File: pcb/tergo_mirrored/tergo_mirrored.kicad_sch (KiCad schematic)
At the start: 111 parts, among them J1 MJ-4PP-9, Q1 2N7002, SW1 SW_RESET, SW10 SW_PUSH, SW11 SW_PUSH, SW12 SW_PUSH, SW13 SW_PUSH, SW14 SW_PUSH, SW15 SW_PUSH, SW16 SW_PUSH, SW17 SW_PUSH, SW18 SW_PUSH, SW19 SW_PUSH, SW2 SW_PUSH, SW20 SW_PUSH, SW21 SW_PUSH, SW22 SW_PUSH, SW23 SW_PUSH, SW24 SW_PUSH, SW25 SW_PUSH, SW26 SW_PUSH, SW27 SW_PUSH, SW28 SW_PUSH, SW29 SW_PUSH, SW3 SW_PUSH, SW4 SW_PUSH, SW5 SW_PUSH, SW6 SW_PUSH, SW7 SW_PUSH, SW8 SW_PUSH, SW9 SW_PUSH, U1 Raspberry_Pi_Pico

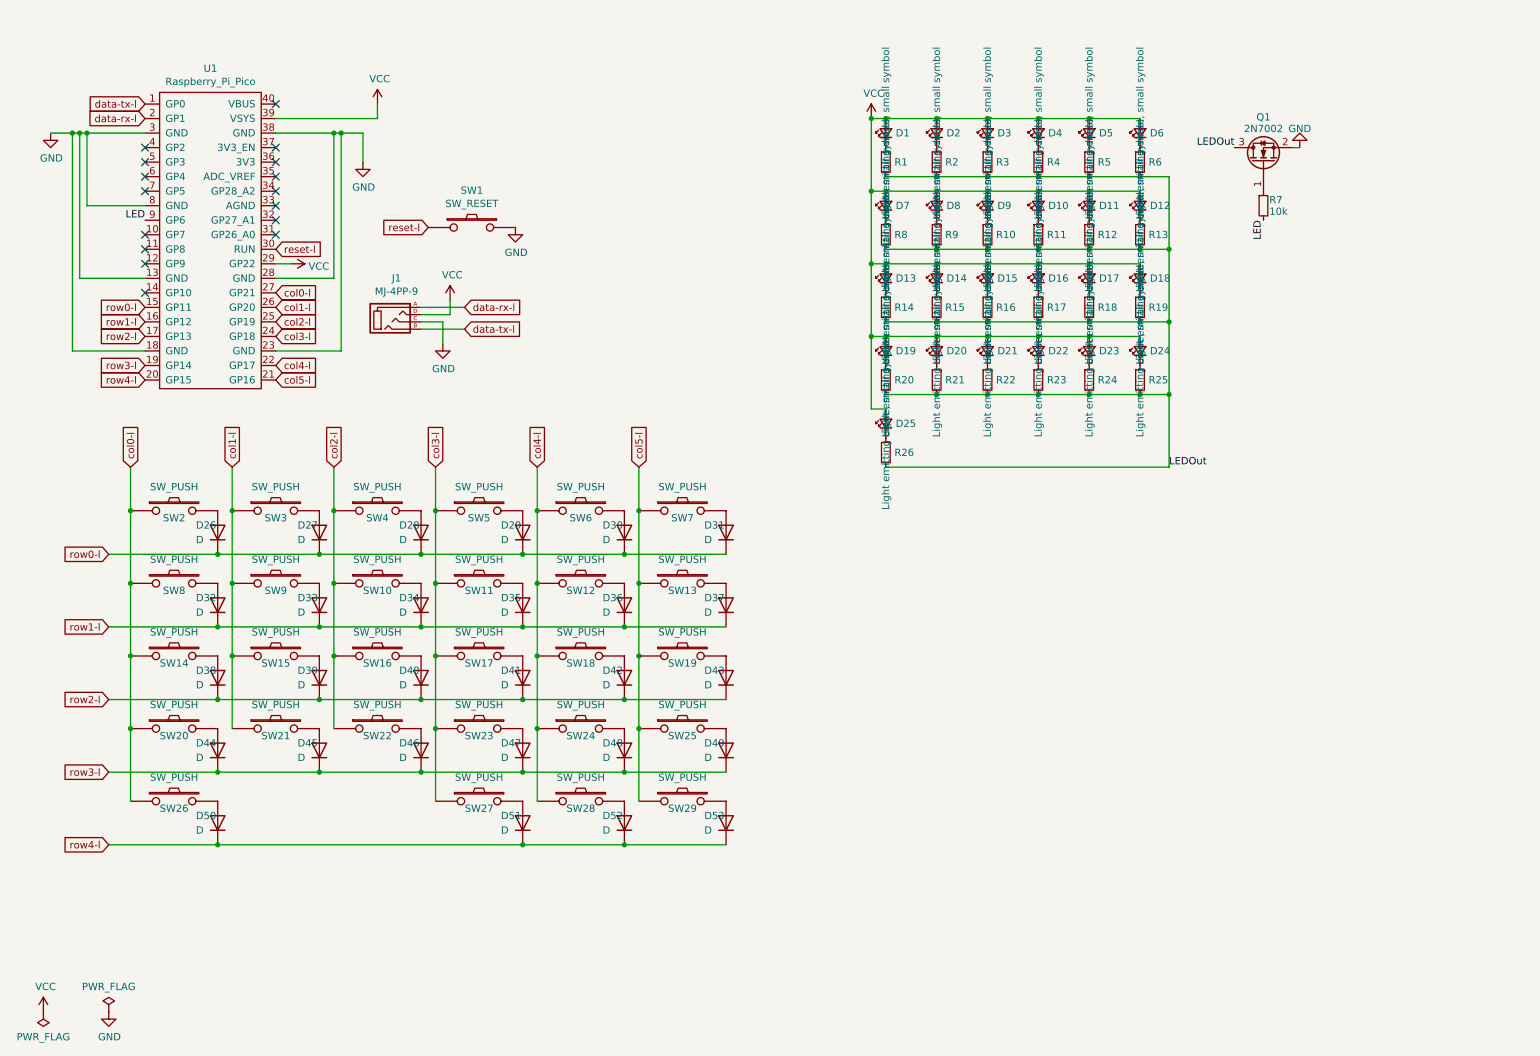
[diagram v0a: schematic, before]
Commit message: wip
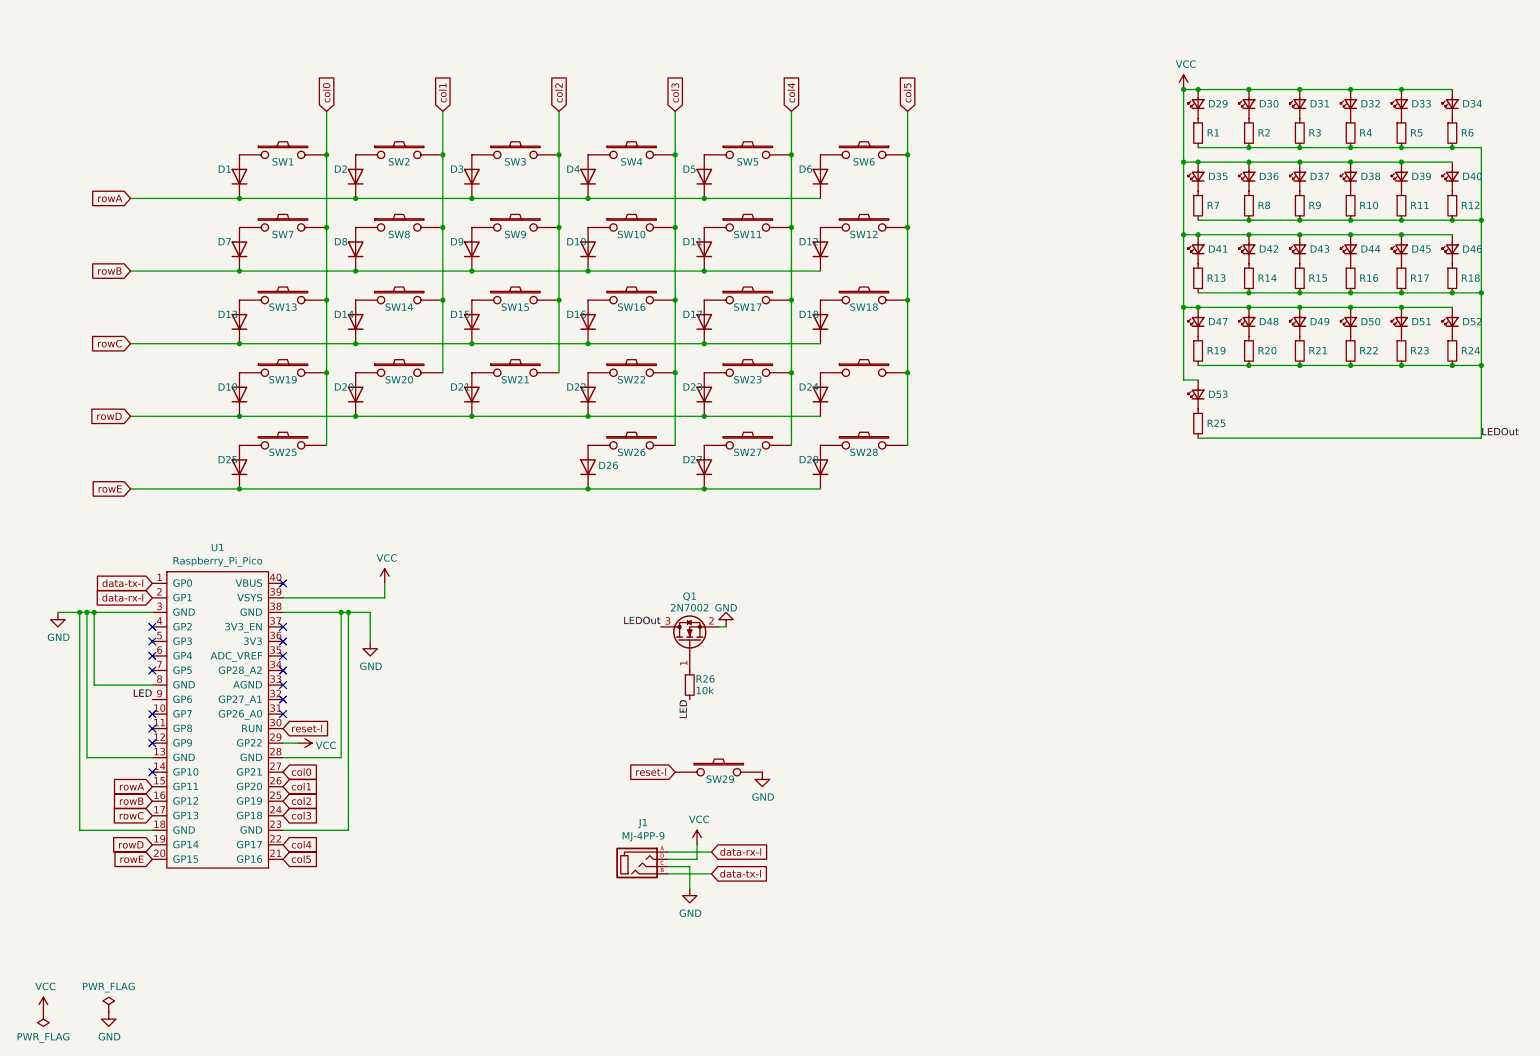
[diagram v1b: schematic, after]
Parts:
- D1: renamed from D26; value D -> 1n4148
- D10: renamed from D35; value D -> 1n4148
- D11: renamed from D36; value D -> 1n4148
- D12: renamed from D37; value D -> 1n4148
- D13: renamed from D38; value D -> 1n4148
- D14: renamed from D39; value D -> 1n4148
- D15: renamed from D40; value D -> 1n4148
- D16: renamed from D41; value D -> 1n4148
- D17: renamed from D42; value D -> 1n4148
- D18: renamed from D43; value D -> 1n4148
- D19: renamed from D44; value D -> 1n4148
- D2: renamed from D27; value D -> 1n4148
- D20: renamed from D45; value D -> 1n4148
- D21: renamed from D46; value D -> 1n4148
- D22: renamed from D47; value D -> 1n4148
- D23: renamed from D48; value D -> 1n4148
- D24: renamed from D49; value D -> 1n4148
- D25: renamed from D50; value D -> 1n4148
- D26: renamed from D51; value D -> 1n4148
- D27: renamed from D52; value D -> 1n4148
- D28: renamed from D53; value D -> 1n4148
- D3: renamed from D28; value D -> 1n4148
- D4: renamed from D29; value D -> 1n4148
- D5: renamed from D30; value D -> 1n4148
- D6: renamed from D31; value D -> 1n4148
- D7: renamed from D32; value D -> 1n4148
- D8: renamed from D33; value D -> 1n4148
- D9: renamed from D34; value D -> 1n4148
- SW1: renamed from SW2; footprint _tergo_lib:CherryMX_Choco_Hotswap -> _tergo_lib:SW_Hotswap_Kailh_MX_Plated_mirrored2_1.00u
- SW10: renamed from SW11; footprint _tergo_lib:CherryMX_Choco_Hotswap -> _tergo_lib:SW_Hotswap_Kailh_MX_Plated_mirrored2_1.00u
- SW11: renamed from SW12; footprint _tergo_lib:CherryMX_Choco_Hotswap -> _tergo_lib:SW_Hotswap_Kailh_MX_Plated_mirrored2_1.00u
- SW12: renamed from SW13; footprint _tergo_lib:CherryMX_Choco_Hotswap -> _tergo_lib:SW_Hotswap_Kailh_MX_Plated_mirrored2_1.00u
- SW13: renamed from SW14; footprint _tergo_lib:CherryMX_Choco_Hotswap -> _tergo_lib:SW_Hotswap_Kailh_MX_Plated_mirrored2_1.00u
- SW14: renamed from SW15; footprint _tergo_lib:CherryMX_Choco_Hotswap -> _tergo_lib:SW_Hotswap_Kailh_MX_Plated_mirrored2_1.00u
- SW15: renamed from SW16; footprint _tergo_lib:CherryMX_Choco_Hotswap -> _tergo_lib:SW_Hotswap_Kailh_MX_Plated_mirrored2_1.00u
- SW16: renamed from SW17; footprint _tergo_lib:CherryMX_Choco_Hotswap -> _tergo_lib:SW_Hotswap_Kailh_MX_Plated_mirrored2_1.00u
- SW17: renamed from SW18; footprint _tergo_lib:CherryMX_Choco_Hotswap -> _tergo_lib:SW_Hotswap_Kailh_MX_Plated_mirrored2_1.00u
- SW18: renamed from SW19; footprint _tergo_lib:CherryMX_Choco_Hotswap -> _tergo_lib:SW_Hotswap_Kailh_MX_Plated_mirrored2_1.00u
- SW19: renamed from SW20; footprint _tergo_lib:CherryMX_Choco_Hotswap -> _tergo_lib:SW_Hotswap_Kailh_MX_Plated_mirrored2_1.00u
- SW2: renamed from SW3; footprint _tergo_lib:CherryMX_Choco_Hotswap -> _tergo_lib:SW_Hotswap_Kailh_MX_Plated_mirrored2_1.00u
- SW20: renamed from SW21; footprint _tergo_lib:CherryMX_Choco_Hotswap -> _tergo_lib:SW_Hotswap_Kailh_MX_Plated_mirrored2_1.00u
- SW21: renamed from SW22; footprint _tergo_lib:CherryMX_Choco_Hotswap -> _tergo_lib:SW_Hotswap_Kailh_MX_Plated_mirrored2_1.00u
- SW22: renamed from SW23; footprint _tergo_lib:CherryMX_Choco_Hotswap -> _tergo_lib:SW_Hotswap_Kailh_MX_Plated_mirrored2_1.00u
- SW23: renamed from SW24; footprint _tergo_lib:CherryMX_Choco_Hotswap -> _tergo_lib:SW_Hotswap_Kailh_MX_Plated_mirrored2_1.00u
- SW24: renamed from SW25; footprint _tergo_lib:CherryMX_Choco_Hotswap -> _tergo_lib:SW_Hotswap_Kailh_MX_Plated_mirrored2_1.00u
- SW25: renamed from SW26; footprint _tergo_lib:CherryMX_Choco_Hotswap -> _tergo_lib:SW_Hotswap_Kailh_MX_Plated_mirrored2_1.00u
- SW26: renamed from SW27; footprint _tergo_lib:CherryMX_Choco_Hotswap -> _tergo_lib:SW_Hotswap_Kailh_MX_Plated_mirrored2_1.00u
- SW27: renamed from SW28; footprint _tergo_lib:CherryMX_Choco_Hotswap -> _tergo_lib:SW_Hotswap_Kailh_MX_Plated_mirrored2_1.00u
- SW28: renamed from SW29; footprint _tergo_lib:CherryMX_Choco_Hotswap -> _tergo_lib:SW_Hotswap_Kailh_MX_Plated_mirrored2_1.00u
- SW29: renamed from SW1; value SW_RESET -> SW_PUSH
- SW3: renamed from SW4; footprint _tergo_lib:CherryMX_Choco_Hotswap -> _tergo_lib:SW_Hotswap_Kailh_MX_Plated_mirrored2_1.00u
- SW4: renamed from SW5; footprint _tergo_lib:CherryMX_Choco_Hotswap -> _tergo_lib:SW_Hotswap_Kailh_MX_Plated_mirrored2_1.00u
- SW5: renamed from SW6; footprint _tergo_lib:CherryMX_Choco_Hotswap -> _tergo_lib:SW_Hotswap_Kailh_MX_Plated_mirrored2_1.00u
- SW6: renamed from SW7; footprint _tergo_lib:CherryMX_Choco_Hotswap -> _tergo_lib:SW_Hotswap_Kailh_MX_Plated_mirrored2_1.00u
- SW7: renamed from SW8; footprint _tergo_lib:CherryMX_Choco_Hotswap -> _tergo_lib:SW_Hotswap_Kailh_MX_Plated_mirrored2_1.00u
- SW8: renamed from SW9; footprint _tergo_lib:CherryMX_Choco_Hotswap -> _tergo_lib:SW_Hotswap_Kailh_MX_Plated_mirrored2_1.00u
- SW9: renamed from SW10; footprint _tergo_lib:CherryMX_Choco_Hotswap -> _tergo_lib:SW_Hotswap_Kailh_MX_Plated_mirrored2_1.00u
- renumbered D1 to D29, D2 to D30, D3 to D31, D4 to D32, D5 to D33, D6 to D34, D7 to D35, D8 to D36, D9 to D37, D10 to D38, D11 to D39, D12 to D40, D13 to D41, D14 to D42, D15 to D43, D16 to D44, D17 to D45, D18 to D46, D19 to D47, D20 to D48, D21 to D49, D22 to D50, D23 to D51, D24 to D52, D25 to D53, R11 to R10, R12 to R11, R13 to R12, R14 to R13, R15 to R14, R16 to R15, R17 to R16, R18 to R17, R19 to R18, R20 to R19, R21 to R20, R22 to R21, R23 to R22, R24 to R23, R25 to R24, R26 to R25, R7 to R26, R8 to R7, R9 to R8, R10 to R9
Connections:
- net at D7.2 (A): now also SW7.1; no longer SW7.2
- net at D13.2 (A): now also SW13.1; no longer SW13.2
- net at D19.2 (A): now also SW19.1; no longer SW19.2
- net at D8.2 (A): now also SW8.1; no longer SW8.2
- net at D14.2 (A): now also SW14.1; no longer SW14.2
- net at D20.2 (A): now also SW20.1; no longer SW20.2
- net at D9.2 (A): now also SW9.1; no longer SW9.2
- net at D15.2 (A): now also SW15.1; no longer SW15.2
- net at D21.2 (A): now also SW21.1; no longer SW21.2
- net at D25.2 (A): now also SW25.1; no longer SW25.2
- net at D10.2 (A): now also SW10.1; no longer SW10.2
- net at D16.2 (A): now also SW16.1; no longer SW16.2
- net at D22.2 (A): now also SW22.1; no longer SW22.2
- net at D26.2 (A): now also SW26.1; no longer SW26.2
- net at D11.2 (A): now also SW11.1; no longer SW11.2
- net at D17.2 (A): now also SW17.1; no longer SW17.2
- net at D23.2 (A): now also SW23.1; no longer SW23.2
- net at D27.2 (A): now also SW27.1; no longer SW27.2
- net at D12.2 (A): now also SW12.1; no longer SW12.2
- net at D18.2 (A): now also SW18.1; no longer SW18.2
- net at D24.2 (A): now also SW24.1; no longer SW24.2
- net at D28.2 (A): now also SW28.1; no longer SW28.2
- net at D3.2 (A): now also SW3.1; no longer SW3.2
- net at D5.2 (A): now also SW5.1; no longer SW5.2
- net at D1.2 (A): now also SW1.1; no longer SW1.2
- net at D2.2 (A): now also SW2.1; no longer SW2.2
- net at D4.2 (A): now also SW4.1; no longer SW4.2
- removed net col0-l: SW1.1, SW13.1, SW19.1, SW25.1, SW7.1, U1.27 (GP21)
- removed net col1-l: SW14.1, SW2.1, SW20.1, SW8.1, U1.26 (GP20)
- removed net col2-l: SW15.1, SW21.1, SW3.1, SW9.1, U1.25 (GP19)
- removed net col3-l: SW10.1, SW16.1, SW22.1, SW26.1, SW4.1, U1.24 (GP18)
- removed net col4-l: SW11.1, SW17.1, SW23.1, SW27.1, SW5.1, U1.22 (GP17)
- removed net col5-l: SW12.1, SW18.1, SW24.1, SW28.1, SW6.1, U1.21 (GP16)
- net row0-l renamed rowA
- net row1-l renamed rowB
- net row2-l renamed rowC
- net row3-l renamed rowD
- net row4-l renamed rowE
- new net col0: SW1.2, SW13.2, SW19.2, SW25.2, SW7.2, U1.27 (GP21)
- new net col1: SW14.2, SW2.2, SW20.2, SW8.2, U1.26 (GP20)
- new net col2: SW15.2, SW21.2, SW3.2, SW9.2, U1.25 (GP19)
- new net col3: SW10.2, SW16.2, SW22.2, SW26.2, SW4.2, U1.24 (GP18)
- new net col4: SW11.2, SW17.2, SW23.2, SW27.2, SW5.2, U1.22 (GP17)
- new net col5: SW12.2, SW18.2, SW24.2, SW28.2, SW6.1, U1.21 (GP16)
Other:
- moved on the sheet: D1, D10, D11, D12, D13, D14, D15, D16, D17, D18, D19, D2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
